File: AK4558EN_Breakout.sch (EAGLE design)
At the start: 35 parts, among them U1 AK4558QFN28

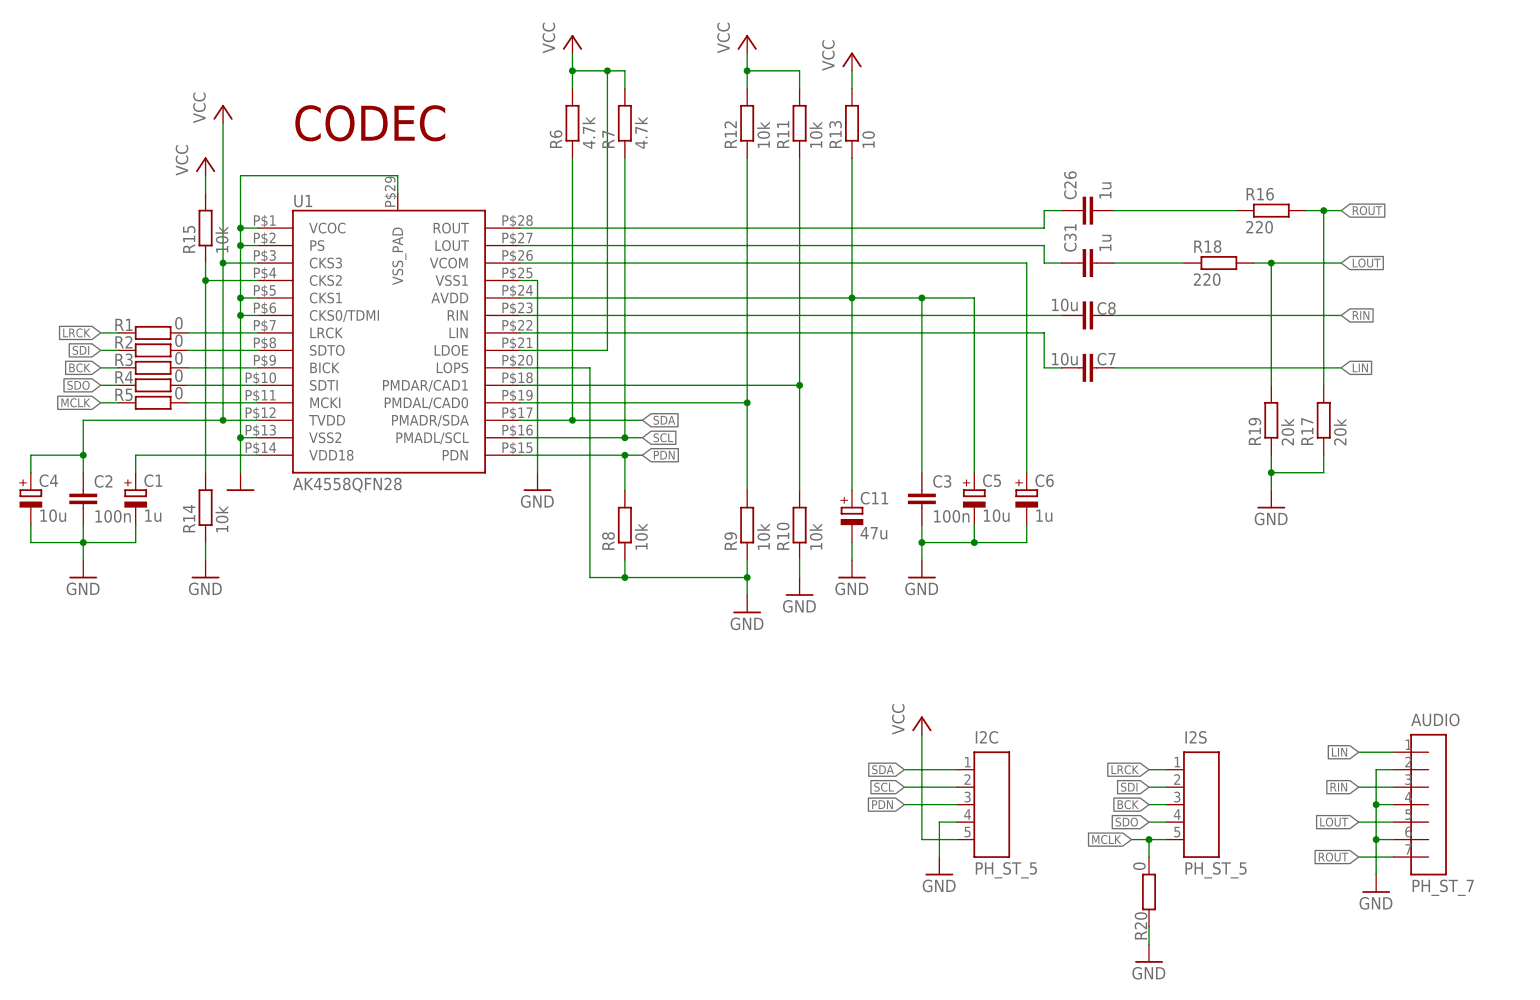
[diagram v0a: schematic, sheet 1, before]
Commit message: update schematic and add gerber
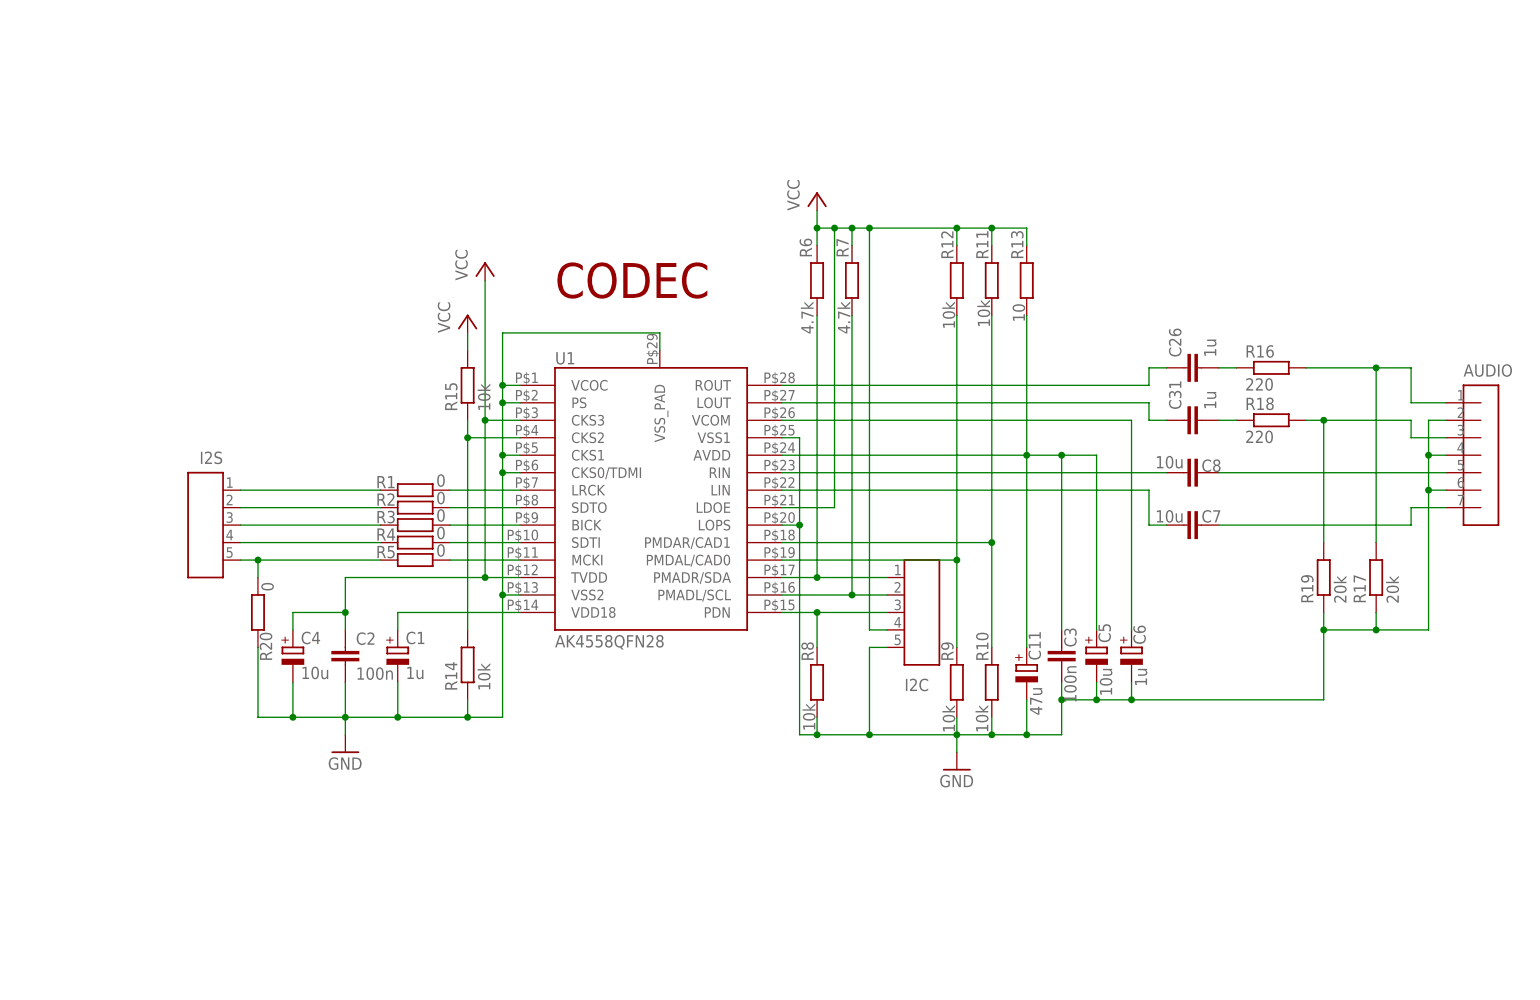
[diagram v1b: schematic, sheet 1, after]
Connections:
- net BCK renamed N$12
- net LRCK renamed N$14
- net SDI renamed N$13
- net SDO renamed N$1
- net GND: now also I2C.P$9; no longer I2C.P$7
- net LIN: now also AUDIO.P$7; no longer AUDIO.P$1
- net LOUT: now also AUDIO.P$3; no longer AUDIO.P$5
- net RIN: now also AUDIO.P$5; no longer AUDIO.P$3
- net ROUT: now also AUDIO.P$1; no longer AUDIO.P$7
- net VCC: now also I2C.P$7; no longer I2C.P$9
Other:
- moved on the sheet: AUDIO, C1, C11, C2, C26, C3, C31, C4, C5, C6, C7, C8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
